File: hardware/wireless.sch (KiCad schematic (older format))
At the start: 14 parts, among them U1 ap6255, U2 SIT1532, Y1 Crystal_GND24

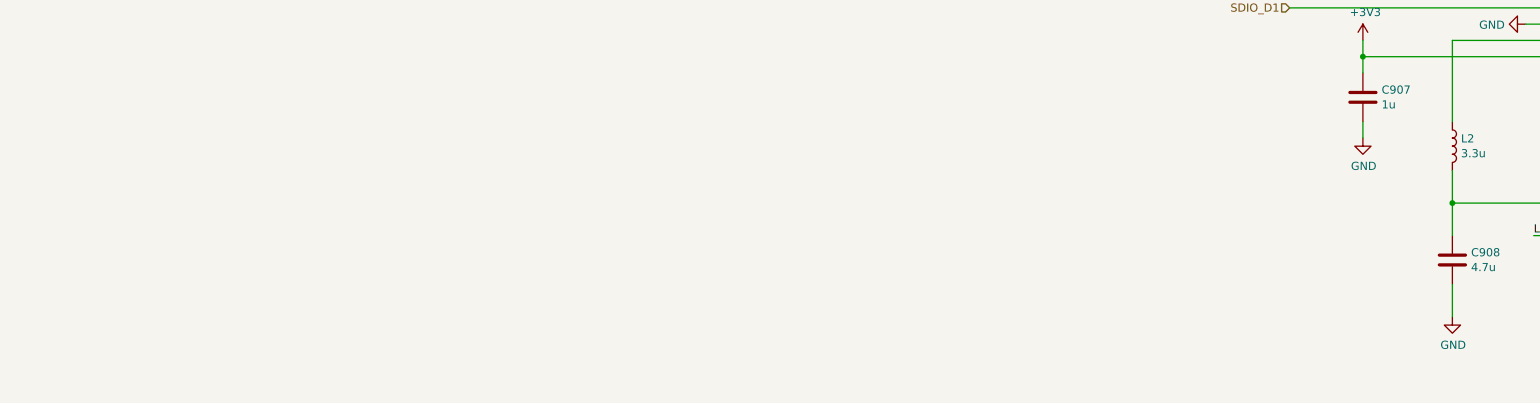
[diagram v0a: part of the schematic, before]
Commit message: wip
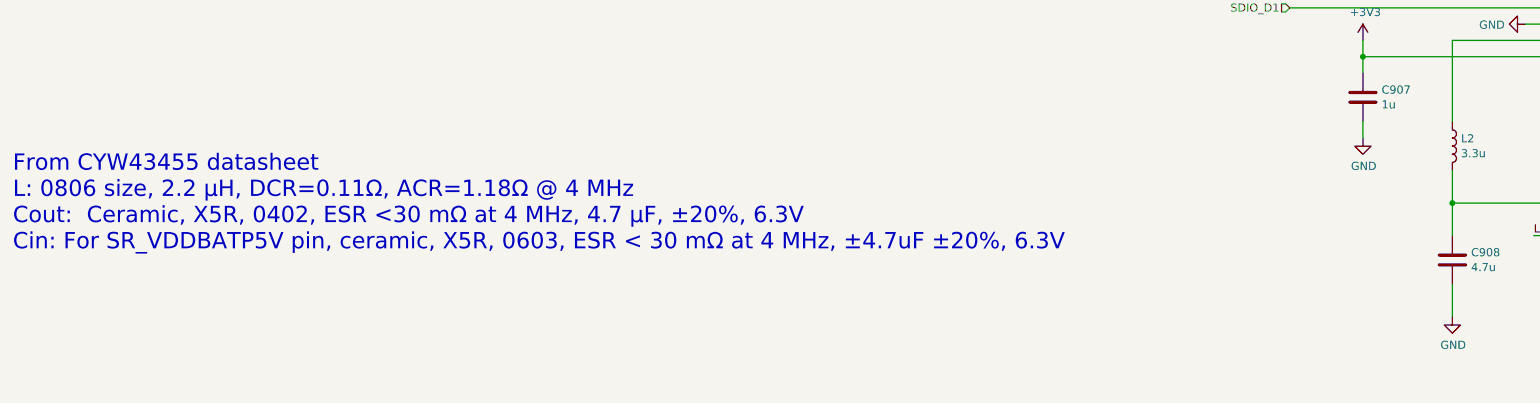
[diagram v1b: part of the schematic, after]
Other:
- note added: "From CYW43455 datasheet\nL: 0806 size, 2.2 µH, DCR=0.11Ω, ACR=1.18Ω @ 4 MHz\nCout: Ceramic, X5R, 0402, ESR <30 mΩ at 4 MHz, 4.7 µF, ±20%, 6.3V\nCin: For SR_VDDBATP5V pin, ceramic, X5R, 0603, ESR < 30 mΩ at 4 MHz, ±4.7uF ±20%, 6.3V"
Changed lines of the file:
@@
 	10100 2800 10100 3100
 Wire Wire Line
-	10100 3100 10550 3100
-Wire Wire Line
 	10100 2800 12150 2800
-Wire Wire Line
-	10850 3100 11100 3100
 Text Notes 10900 2950 0    50   ~ 0
 epson fa-128
@@
 	1    0    0    -1
 $EndComp
+Text Notes 1850 6150 0    100  ~ 0
+From CYW43455 datasheet\nL: 0806 size, 2.2 µH, DCR=0.11Ω, ACR=1.18Ω @ 4 MHz\nCout:  Ceramic, X5R, 0402, ESR <30 mΩ at 4 MHz, 4.7 µF, ±20%, 6.3V\nCin: For SR_VDDBATP5V pin, ceramic, X5R, 0603, ESR < 30 mΩ at 4 MHz, ±4.7uF ±20%, 6.3V
+Wire Wire Line
+	10100 3100 10550 3100
+Wire Wire Line
+	10850 3100 11100 3100
 $EndSCHEMATC
